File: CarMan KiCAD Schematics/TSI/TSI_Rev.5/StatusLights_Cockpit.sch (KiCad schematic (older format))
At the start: 18 parts, among them Q3 ZVP1320F, U1 RDE03110S12, U11 TLP293, U13 TLP293

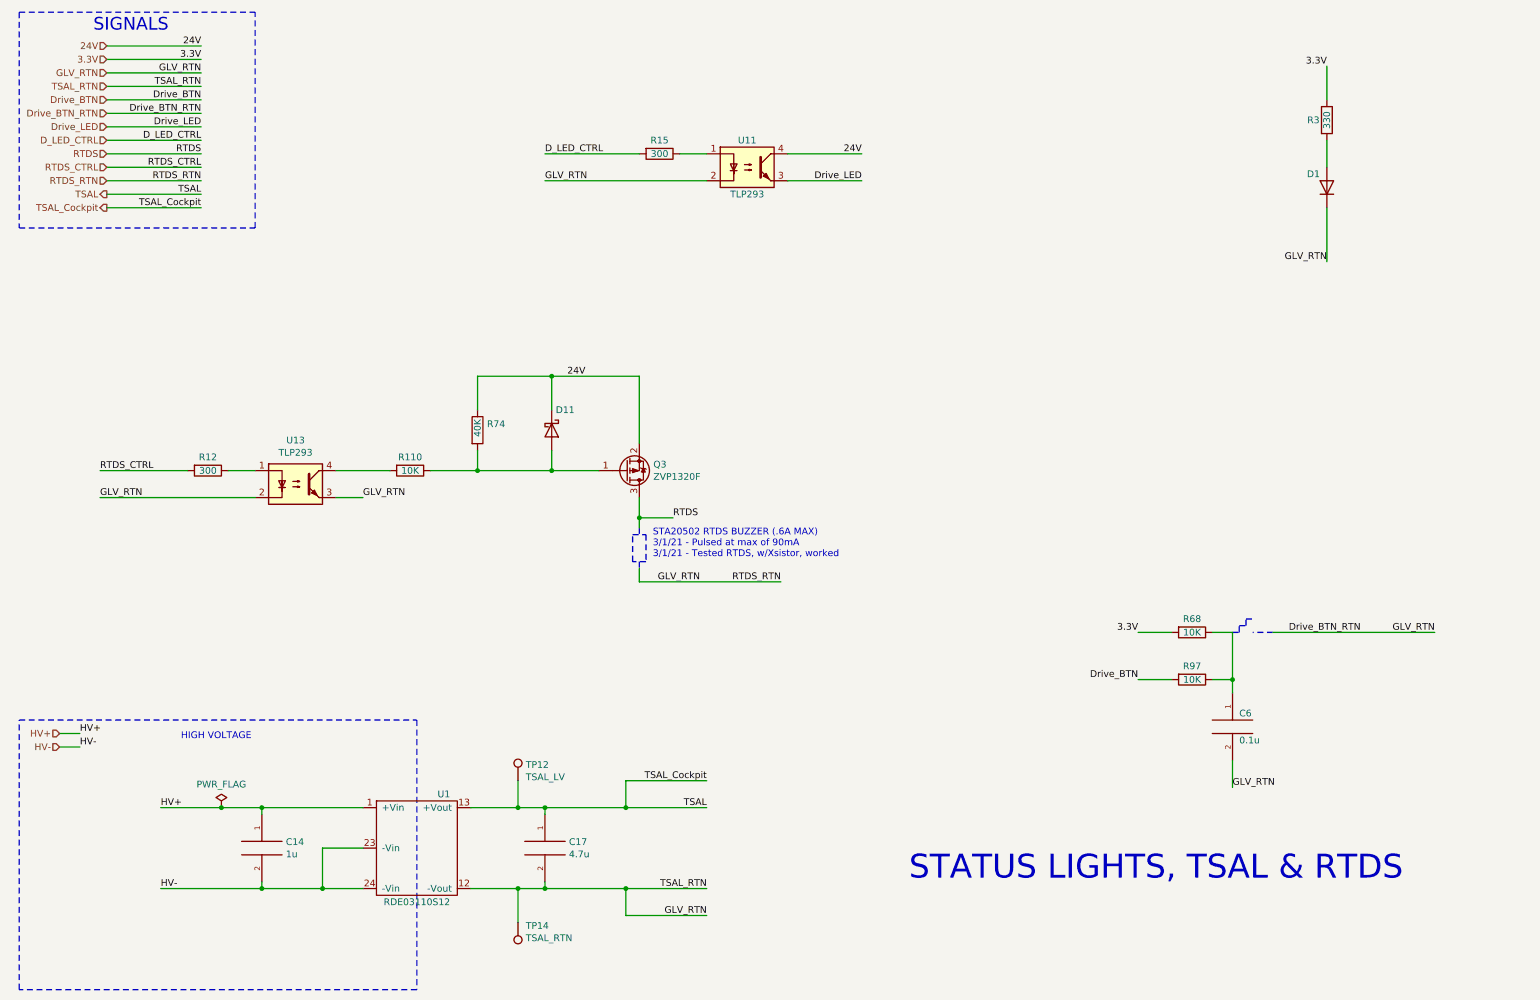
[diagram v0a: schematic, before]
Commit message: Organizational
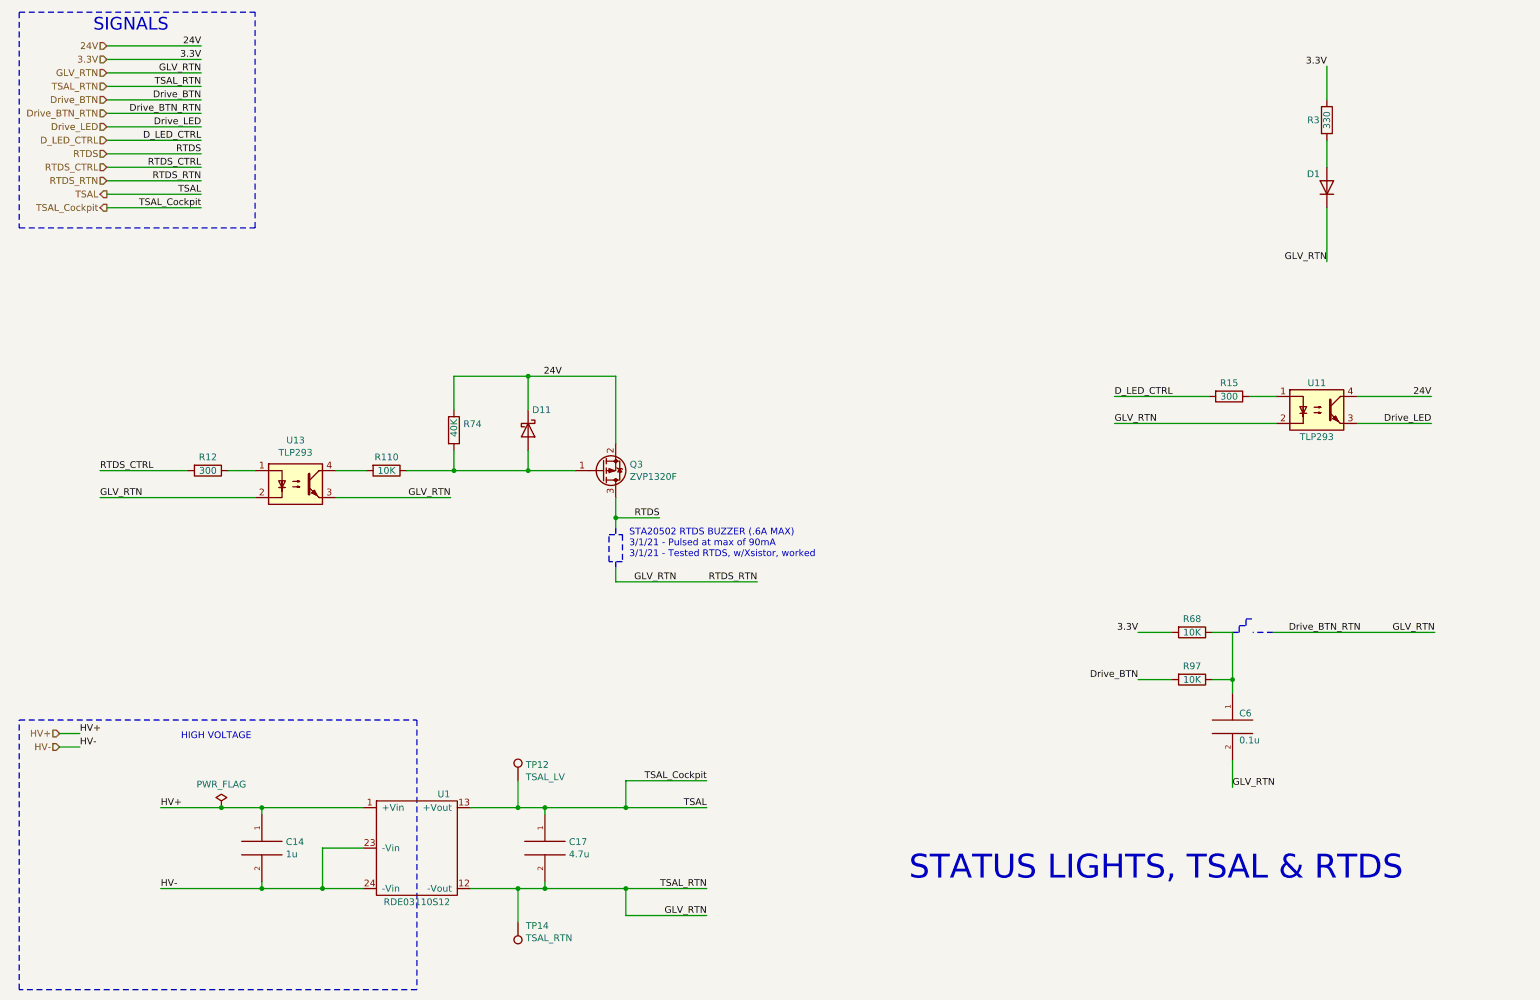
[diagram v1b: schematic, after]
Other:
- moved on the sheet: D11, Q3, R110, R15, R74, U11
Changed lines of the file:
@@
 $Descr A4 11693 8268
 encoding utf-8
-Sheet 6 6
+Sheet 5 6
 Title ""
 Date ""
@@
 L TSI_Rev.5-rescue:TLP293-CarMan_KiCAD_Library-TSI_Rev.5-rescue U11
 U 1 1 5F9A966C
-P 5900 1650
-F 0 "U11" H 5900 1850 50  0000 C CNN
-F 1 "TLP293" H 5900 1450 50  0000 C CNN
-F 2 "Package_SO:SOIC-4_4.55x2.6mm_P1.27mm" H 5700 1450 50  0001 L CIN
-F 3 "" H 5900 1650 50  0001 L CNN
-	1    5900 1650
+P 10125 3450
+F 0 "U11" H 10125 3650 50  0000 C CNN
+F 1 "TLP293" H 10125 3250 50  0000 C CNN
+F 2 "Package_SO:SOIC-4_4.55x2.6mm_P1.27mm" H 9925 3250 50  0001 L CIN
+F 3 "" H 10125 3450 50  0001 L CNN
+	1    10125 3450
 	1    0    0    -1
 $EndComp
@@
 L Device:R R15
 U 1 1 5F9DEF51
-P 5250 1550
-F 0 "R15" V 5150 1550 50  0000 C CNN
-F 1 "300" V 5250 1550 50  0000 C CNN
-F 2 "Resistor_SMD:R_0805_2012Metric_Pad1.15x1.40mm_HandSolder" V 5180 1550 50  0001 C CNN
-F 3 "~" H 5250 1550 50  0001 C CNN
-	1    5250 1550
+P 9475 3350
+F 0 "R15" V 9375 3350 50  0000 C CNN
+F 1 "300" V 9475 3350 50  0000 C CNN
+F 2 "Resistor_SMD:R_0805_2012Metric_Pad1.15x1.40mm_HandSolder" V 9405 3350 50  0001 C CNN
+F 3 "~" H 9475 3350 50  0001 C CNN
+	1    9475 3350
 	0    1    1    0
 $EndComp
-Text Label 6750 1550 2    50   ~ 0
+Text Label 10975 3350 2    50   ~ 0
 24V
-Text Label 6750 1750 2    50   ~ 0
+Text Label 10975 3550 2    50   ~ 0
 Drive_LED
-Text Label 4400 1750 0    50   ~ 0
-GLV_RTN
-Text Label 4400 1550 0    50   ~ 0
+Text Label 8625 3550 0    50   ~ 0
+GLV_RTN
+Text Label 8625 3350 0    50   ~ 0
 D_LED_CTRL
-Text Label 4700 3200 2    50   ~ 0
+Text Label 4525 3200 2    50   ~ 0
 24V
 Text HLabel 800  5850 0    50   Input ~ 0
@@
 Drive_BTN
 Wire Wire Line
-	5600 1550 5400 1550
+	9825 3350 9625 3350
 Text Notes 7100 6950 0    177  ~ 0
 STATUS LIGHTS, TSAL & RTDS
@@
 	0    1    1    0
 $EndComp
-Connection ~ 4450 3200
-Wire Wire Line
-	4450 3200 5100 3200
-Wire Wire Line
-	3900 3200 4450 3200
+Connection ~ 4275 3200
+Wire Wire Line
+	4275 3200 4925 3200
+Wire Wire Line
+	3725 3200 4275 3200
 $Comp
 L CarMan_KiCAD_Library:D_Schottky D11
 U 1 1 5F9B6857
-P 4450 3600
-F 0 "D11" V 4300 3700 50  0000 C CNN
-F 1 "MMSZ5231B-7-F" H 4450 3726 50  0001 C CNN
-F 2 "Diode_SMD:D_SOD-123" H 4450 3600 50  0001 C CNN
-F 3 "~" H 4450 3600 50  0001 C CNN
-	1    4450 3600
+P 4275 3600
+F 0 "D11" V 4125 3700 50  0000 C CNN
+F 1 "MMSZ5231B-7-F" H 4275 3726 50  0001 C CNN
+F 2 "Diode_SMD:D_SOD-123" H 4275 3600 50  0001 C CNN
+F 3 "~" H 4275 3600 50  0001 C CNN
+	1    4275 3600
 	0    1    1    0
 $EndComp
 Wire Wire Line
-	5100 4725 6150 4725
-Wire Wire Line
-	4450 3900 4800 3900
+	4925 4725 5975 4725
+Wire Wire Line
+	4275 3900 4625 3900
 $Comp
 L Device:Q_PMOS_GSD Q?
 U 1 1 5FC93215
-P 5000 3900
+P 4825 3900
 AR Path="/6196BF15/5FC93215" Ref="Q?"  Part="1"
 AR Path="/5FE1DCBA/5FC93215" Ref="Q3"  Part="1"
-F 0 "Q3" H 5204 3854 50  0000 L CNN
-F 1 "ZVP1320F" H 5204 3945 50  0000 L CNN
-F 2 "TSI_Rev_2021_Footprint_Lib:SOT23" H 5200 4000 50  0001 C CNN
-F 3 "https://www.snapeda.com/parts/ZVP1320FTA/Diodes%20Inc./datasheet/" H 5000 3900 50  0001 C CNN
-	1    5000 3900
+F 0 "Q3" H 5029 3854 50  0000 L CNN
+F 1 "ZVP1320F" H 5029 3945 50  0000 L CNN
+F 2 "TSI_Rev_2021_Footprint_Lib:SOT23" H 5025 4000 50  0001 C CNN
+F 3 "https://www.snapeda.com/parts/ZVP1320FTA/Diodes%20Inc./datasheet/" H 4825 3900 50  0001 C CNN
+	1    4825 3900
 	1    0    0    1
 $EndComp
 Wire Wire Line
-	3050 4100 2850 4100
-Wire Wire Line
 	2250 3900 2050 3900
-Text Notes 5200 4550 0    50   ~ 0
+Text Notes 5025 4550 0    50   ~ 0
 STA20502 RTDS BUZZER (.6A MAX)\n3/1/21 - Pulsed at max of 90mA\n3/1/21 - Tested RTDS, w/Xsistor, worked\n
 Wire Notes Line
-	5100 4575 5100 4625
-Wire Notes Line
-	5050 4375 5150 4375
-Wire Notes Line
-	5050 4575 5050 4375
-Wire Notes Line
-	5150 4575 5050 4575
-Wire Notes Line
-	5150 4375 5150 4575
-Wire Notes Line
-	5100 4325 5100 4375
-Text Label 5550 4725 2    50   ~ 0
-GLV_RTN
-Text Label 6150 4725 2    50   ~ 0
+	4925 4575 4925 4625
+Wire Notes Line
+	4875 4375 4975 4375
+Wire Notes Line
+	4875 4575 4875 4375
+Wire Notes Line
+	4975 4575 4875 4575
+Wire Notes Line
+	4975 4375 4975 4575
+Wire Notes Line
+	4925 4325 4925 4375
+Text Label 5375 4725 2    50   ~ 0
+GLV_RTN
+Text Label 5975 4725 2    50   ~ 0
 RTDS_RTN
-Text Label 5350 4250 0    50   ~ 0
+Text Label 5250 4250 2    50   ~ 0
 RTDS
 Wire Wire Line
-	5100 4250 5350 4250
-Wire Wire Line
-	5100 4100 5100 4250
-Connection ~ 4450 3900
-Wire Wire Line
-	5100 3200 5100 3700
-Text Label 3050 4100 0    50   ~ 0
+	4925 4100 4925 4250
+Connection ~ 4275 3900
+Wire Wire Line
+	4925 3200 4925 3700
+Text Label 3700 4100 2    50   ~ 0
 GLV_RTN
 $Comp
@@
 $EndComp
 Wire Wire Line
-	4450 3450 4450 3200
-Wire Wire Line
-	3900 3450 3900 3200
-Connection ~ 3900 3900
-Wire Wire Line
-	4450 3900 4450 3750
-Wire Wire Line
-	3900 3900 4450 3900
-Wire Wire Line
-	3900 3900 3900 3750
-Wire Wire Line
-	3550 3900 3900 3900
-Wire Wire Line
-	2850 3900 3250 3900
+	4275 3450 4275 3200
+Wire Wire Line
+	3725 3450 3725 3200
+Connection ~ 3725 3900
+Wire Wire Line
+	4275 3900 4275 3750
+Wire Wire Line
+	3725 3900 4275 3900
+Wire Wire Line
+	3725 3900 3725 3750
+Wire Wire Line
+	3375 3900 3725 3900
 $Comp
 L Device:R R74
 U 1 1 5F9BC6E2
-P 3900 3600
-F 0 "R74" H 3970 3646 50  0000 L CNN
-F 1 "40K" V 3900 3550 50  0000 L CNN
-F 2 "Resistor_SMD:R_0805_2012Metric_Pad1.15x1.40mm_HandSolder" V 3830 3600 50  0001 C CNN
-F 3 "~" H 3900 3600 50  0001 C CNN
-	1    3900 3600
+P 3725 3600
+F 0 "R74" H 3795 3646 50  0000 L CNN
+F 1 "40K" V 3725 3550 50  0000 L CNN
+F 2 "Resistor_SMD:R_0805_2012Metric_Pad1.15x1.40mm_HandSolder" V 3655 3600 50  0001 C CNN
+F 3 "~" H 3725 3600 50  0001 C CNN
+	1    3725 3600
 	1    0    0    -1
 $EndComp
@@
 L Device:R R110
 U 1 1 5F9BBE04
-P 3400 3900
-F 0 "R110" V 3300 3900 50  0000 C CNN
-F 1 "10K" V 3400 3900 50  0000 C CNN
-F 2 "Resistor_SMD:R_0805_2012Metric_Pad1.15x1.40mm_HandSolder" V 3330 3900 50  0001 C CNN
-F 3 "~" H 3400 3900 50  0001 C CNN
-	1    3400 3900
+P 3225 3900
+F 0 "R110" V 3125 3900 50  0000 C CNN
+F 1 "10K" V 3225 3900 50  0000 C CNN
+F 2 "Resistor_SMD:R_0805_2012Metric_Pad1.15x1.40mm_HandSolder" V 3155 3900 50  0001 C CNN
+F 3 "~" H 3225 3900 50  0001 C CNN
+	1    3225 3900
 	0    1    1    0
 $EndComp
@@
 	4400 7000 5000 7000
 Wire Wire Line
-	4400 1550 5100 1550
-Wire Wire Line
-	4400 1750 5600 1750
-Wire Wire Line
-	6200 1550 6750 1550
-Wire Wire Line
-	6200 1750 6750 1750
+	8625 3350 9325 3350
+Wire Wire Line
+	8625 3550 9825 3550
+Wire Wire Line
+	10425 3350 10975 3350
+Wire Wire Line
+	10425 3550 10975 3550
 Wire Notes Line
 	500  2100 2250 2100
@@
 GLV_RTN
 Wire Wire Line
-	5100 4250 5100 4325
-Connection ~ 5100 4250
-Wire Wire Line
-	5100 4625 5100 4725
+	4925 4250 4925 4325
+Connection ~ 4925 4250
+Wire Wire Line
+	4925 4625 4925 4725
+Wire Wire Line
+	4925 4250 5250 4250
+Wire Wire Line
+	2850 3900 3075 3900
+Wire Wire Line
+	2850 4100 3700 4100
 $EndSCHEMATC
